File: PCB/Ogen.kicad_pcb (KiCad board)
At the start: 2 copper layers, 28 x 21.5 mm, 17 parts, among them J1 Input, U1 PMW3360DM-T2QU, U2 TLV70019, U3 TXS0102DCU, U4 TXS0102DCU, U5 TXS0102DCU

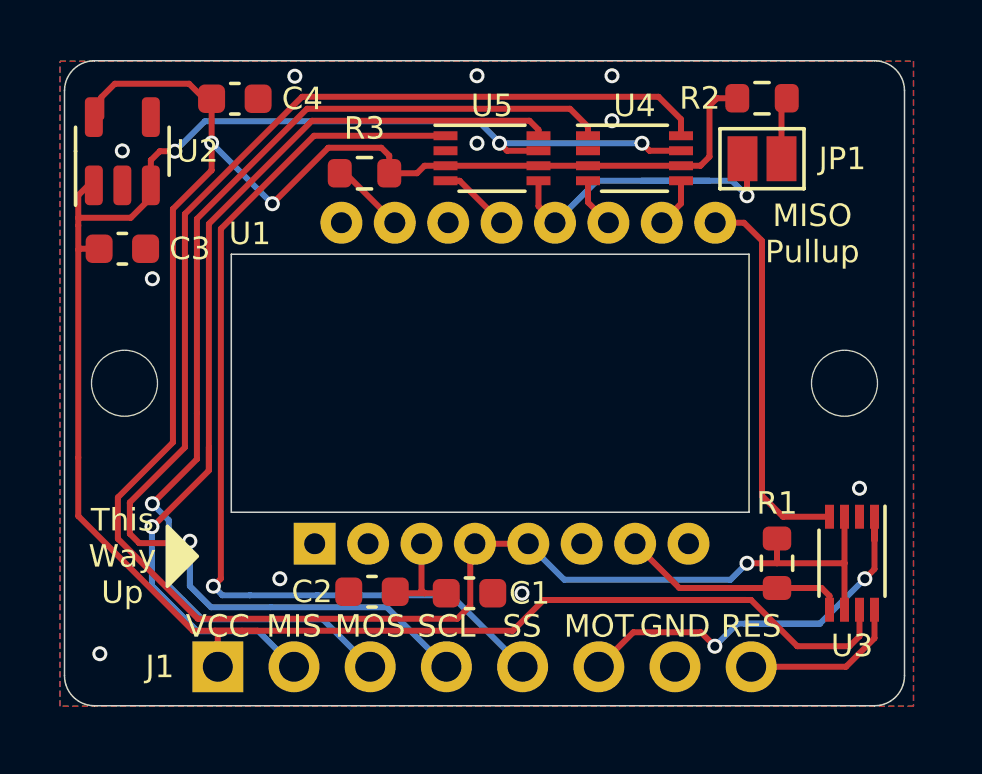
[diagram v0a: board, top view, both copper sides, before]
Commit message: V1.0 Lite initial commit.
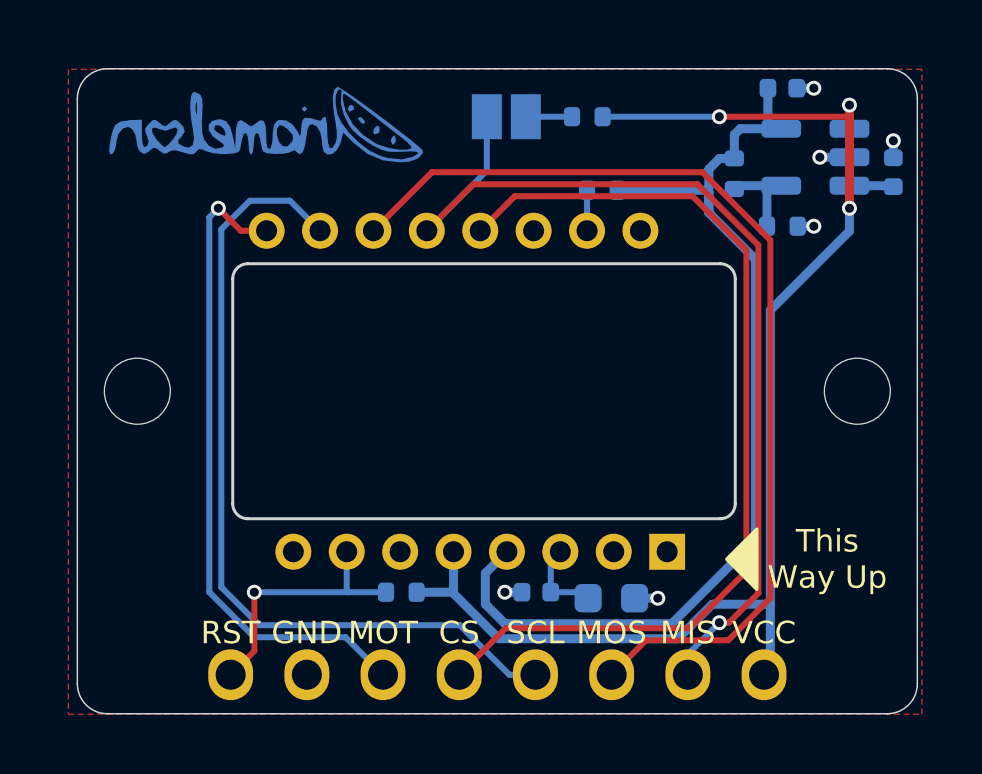
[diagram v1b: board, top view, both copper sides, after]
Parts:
- removed U3, U4, U5: TXS0102DCU, Package_SO:VSSOP-8_2.3x2mm_P0.5mm
- added R4: 10k, Resistor_SMD:R_0402_1005Metric, B.Cu at (36.5, 18.5)
- added R5: 15k, Resistor_SMD:R_0402_1005Metric, B.Cu at (34.9, 16.7)
- A1: footprint Ogen:Ariamelon_Logo -> Ogen:Ariamelon_Logo-CU
- C1: value 4.7uF -> 1u; footprint Capacitor_SMD:C_0603_1608Metric -> Capacitor_SMD:C_0402_1005Metric; moved to B.Cu
- C2: value 100nF -> 4u7; moved to B.Cu
- C3: value 1uF -> 100n; footprint Capacitor_SMD:C_0603_1608Metric -> Capacitor_SMD:C_0402_1005Metric; moved to B.Cu
- C4: value 1uF -> 1u; footprint Capacitor_SMD:C_0603_1608Metric -> Capacitor_SMD:C_0402_1005Metric; moved to B.Cu
- H1, H2, U1: moved to B.Cu
- J1: footprint Connector_PinHeader_2.54mm:PinHeader_1x08_P2.54mm_Vertical -> Ogen:PinHeader_1x08_P2.54mm_Vertical; moved to B.Cu
- JP1: value Jumper -> MISO_Pullup; moved to B.Cu
- R1: footprint Resistor_SMD:R_0603_1608Metric -> Resistor_SMD:R_0402_1005Metric; moved to B.Cu
- R2: value 10k -> 39; footprint Resistor_SMD:R_0603_1608Metric -> Resistor_SMD:R_0402_1005Metric; moved to B.Cu
- R3: value 39R -> 10k; footprint Resistor_SMD:R_0603_1608Metric -> Resistor_SMD:R_0402_1005Metric; moved to B.Cu
- U2: value TLV70019 -> AP2127K-ADJ; moved to B.Cu
- moved H1 24.4 mm to (39.0, 24.0)
- moved H2 23.6 mm to (15.0, 24.0)
- moved U2 23.1 mm to (37.6, 16.2), turned to 180 degrees
- moved C1 19.9 mm to (40.2, 16.7), turned to 90 degrees
- moved C4 18.3 mm to (36.5, 13.9)
- moved C3 17.9 mm to (28.3, 30.7)
- moved R1 12.6 mm to (23.8, 30.7), turned to 0 degrees
- moved J1 9.32 mm to (35.9, 33.5)
- moved JP1 8.64 mm to (27.3, 14.9)
- moved A1 8.05 mm to (19.3, 15.1)
- moved C2 7.98 mm to (30.8, 30.9), turned to 0 degrees
- moved R3 7.66 mm to (30.0, 14.8)
- moved R2 6.14 mm to (30.5, 17.3), turned to 0 degrees
- moved U1 0.50 mm to (27.0, 24.0)
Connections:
- C1 pad 1: Net-(C1-Pad1) -> +3V3
- C2 pad 1: Net-(C1-Pad1) -> Net-(U1-VDDPIX)
- C3 pad 1: VCC -> GND
- C3 pad 2: GND -> Net-(U1-VDDPIX)
- C4 pad 1: VDD -> +2V
- J1 pad 1: VCC -> +3V3
- J1 pad 2: MISO-H -> /MISO
- J1 pad 3: MOSI-H -> /MOSI
- J1 pad 4: SCLK-H -> /SCK
- J1 pad 5: SS-H -> /CS
- J1 pad 6: MOT-H -> /MOTION
- J1 pad 8: NRESET-H -> /~{RST}
- JP1 pad 1: Net-(JP1-Pad1) -> Net-(JP1-A)
- JP1 pad 2: MISO -> /MISO
- R1 pad 1: NRESET -> /~{RST}
- R1 pad 2: VDD -> +3V3
- R2 pad 1: Net-(JP1-Pad1) -> Net-(U1-LED_P)
- R2 pad 2: VDD -> +2V
- R3 pad 1: Net-(R3-Pad1) -> Net-(JP1-A)
- R3 pad 2: VDD -> +3V3
- U1 pad 10: SCLK -> /SCK
- U1 pad 11: MOSI -> /MOSI
- U1 pad 12: MISO -> /MISO
- U1 pad 13: SS -> /CS
- U1 pad 15: Net-(R3-Pad1) -> Net-(U1-LED_P)
- U1 pad 3: Net-(C1-Pad1) -> Net-(U1-VDDPIX)
- U1 pad 4: VDD -> +2V
- U1 pad 5: VDD -> +3V3
- U1 pad 7: NRESET -> /~{RST}
- U1 pad 9: MOT -> /MOTION
- U2 pad 1: VCC -> +3V3
- U2 pad 3: VCC -> +3V3
- U2 pad 4: unconnected-(U2-Pad4) -> Net-(U2-ADJ)
- U2 pad 5: VDD -> +2V
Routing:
- net VDD: track 74.4 -> 0.00 mm, vias 3 -> 0
- net VCC: track 70.0 -> 0.00 mm, vias 3 -> 0
- net +3V3: track 0.00 -> 45.7 mm, vias 0 -> 3
- net SCLK-H: track 43.8 -> 0.00 mm, vias 1 -> 0
- net MOSI-H: track 36.0 -> 0.00 mm, vias 1 -> 0
- net MISO-H: track 34.3 -> 0.00 mm, vias 1 -> 0
- net +2V: track 0.00 -> 34.1 mm
- net /MOSI: track 0.00 -> 33.3 mm
- net /MISO: track 0.00 -> 32.6 mm, vias 0 -> 1
- net SS-H: track 32.2 -> 0.00 mm, vias 1 -> 0
- net /CS: track 0.00 -> 31.8 mm
- net /SCK: track 0.00 -> 27.7 mm
- net /MOTION: track 0.00 -> 21.8 mm, vias 0 -> 1
- net MOT-H: track 16.0 -> 0.00 mm, vias 2 -> 0
- net MOT: track 12.8 -> 0.00 mm
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- removed copper zone on B.Cu, net GND
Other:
- board text added: "CS"
- board text added: "Ogen V1.2"
- board text added: "RST"
- board text removed: "MISO Pullup"
- board text removed: "Ogen V1.1"
- board text removed: "RES"
- board text removed: "SS"
